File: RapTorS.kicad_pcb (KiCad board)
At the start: 2 copper layers, 45 x 19 mm, 23 parts, among them J1 Molex 48037-2200, J2 TestPoint, J3 TestPoint, J4 TestPoint, J5 TestPoint, J6 TestPoint, U1 PIC16LF1454-I_ML, U2 TLV71333PDBV, U3 E07-M1101S

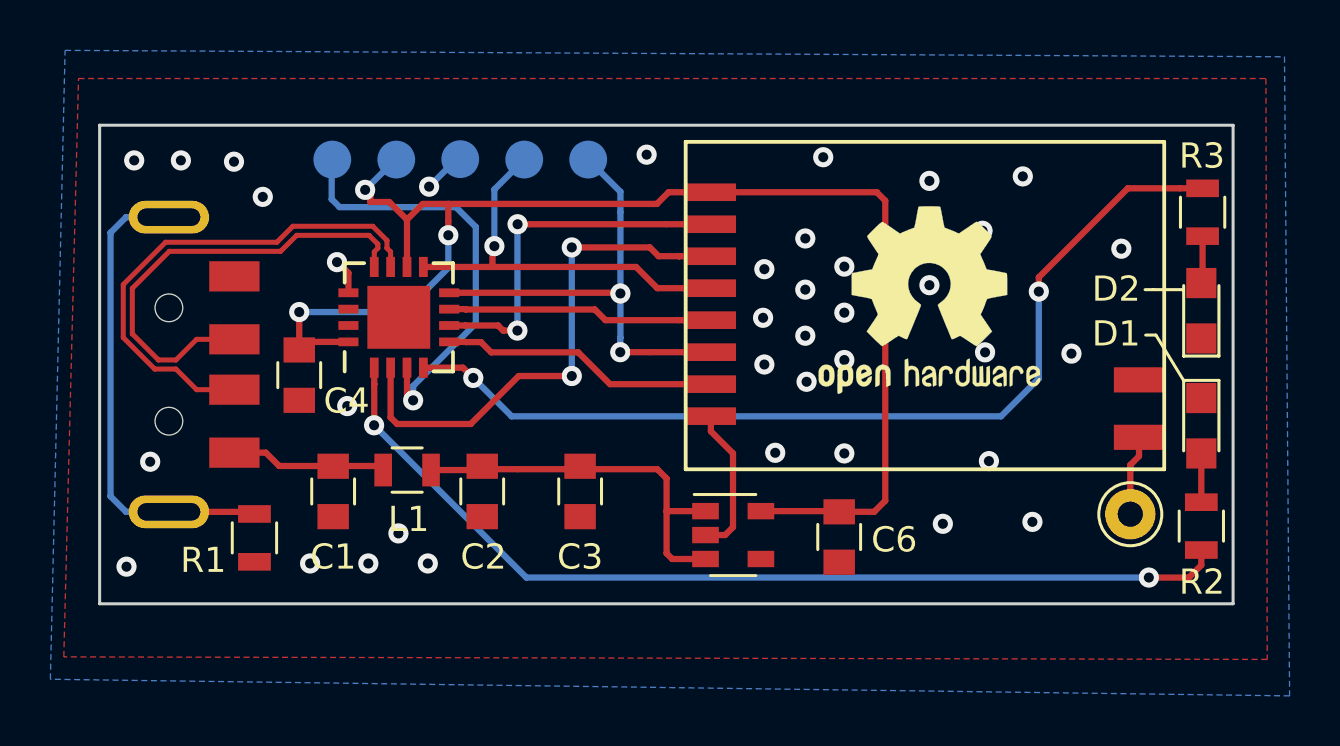
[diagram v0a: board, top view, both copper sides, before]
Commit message: routing completed
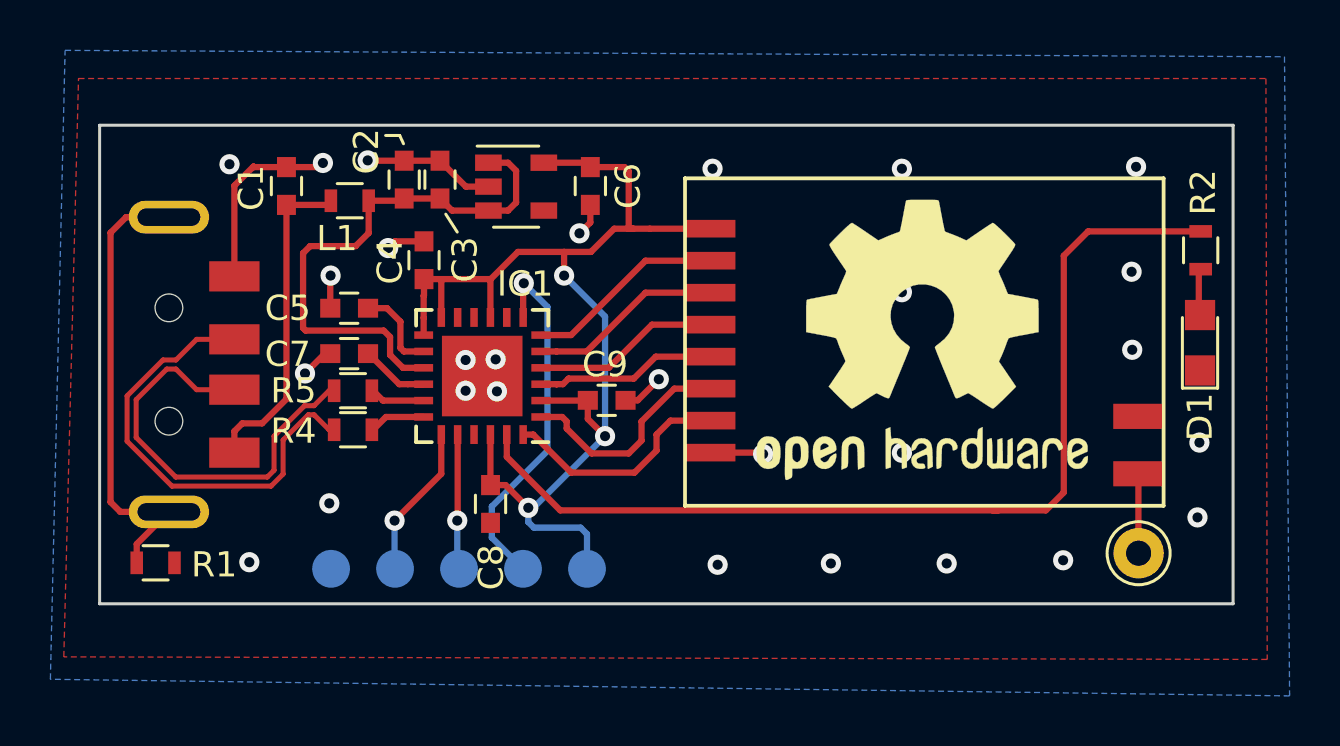
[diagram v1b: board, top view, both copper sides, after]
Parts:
- removed D2: LED_ALT, LEDs:LED_0805
- removed G***: LOGO, Logo:Logo
- removed R3: 50R, Resistors_SMD:R_0805
- removed the REF*** at (171.7, 98.1)
- removed U1: PIC16LF1454-I_ML, Housings_DFN_QFN:QFN-16-1EP_4x4mm_Pitch0.65mm
- added C5: 1uF, Capacitors_SMD:C_0603, F.Cu at (148.7, 98.4)
- added C7: 1uF, Capacitors_SMD:C_0603, F.Cu at (148.7, 100.2)
- added C8: 1uF, Capacitors_SMD:C_0603, F.Cu at (154.3, 106.2)
- added C9: 1uF, Capacitors_SMD:C_0603, F.Cu at (158.9, 102.1)
- added IC1: EFM32HG308F64G-A-QFN24, Housings_DFN_QFN:QFN-24-1EP_5x5mm_Pitch0.65mm, F.Cu at (153.9, 101.1)
- added R4: 15R, Resistors_SMD:R_0603, F.Cu at (148.8, 103.3)
- added R5: 15R, Resistors_SMD:R_0603, F.Cu at (148.8, 101.7)
- added RAPTORS: LOGO, Logo:Logo, B.Cu at (163.1, 100.4)
- added REF***: OSHW-Logo2_14.6x12mm_SilkScreen, Symbols:OSHW-Logo2_14.6x12mm_SilkScreen, F.Cu at (171.4, 99.7)
- C1, C2, C3, C4, C6: footprint Capacitors_SMD:C_0805 -> Capacitors_SMD:C_0603
- L1: footprint Inductors_SMD:L_0805 -> Inductors_SMD:L_0603
- R1, R2: footprint Resistors_SMD:R_0805 -> Resistors_SMD:R_0603
- moved J6 18.0 mm to (150.5, 108.8)
- moved J2 17.9 mm to (155.6, 108.8)
- moved J3 17.9 mm to (158.1, 108.8)
- moved C6 17.1 mm to (158.2, 93.6)
- moved J4 17.1 mm to (147.9, 108.8)
- moved J5 16.5 mm to (153.0, 108.8)
- moved U2 16.3 mm to (155.3, 93.6)
- moved C3 13.6 mm to (152.3, 93.3), turned to 90 degrees
- moved C2 12.8 mm to (150.9, 93.3), turned to 90 degrees
- moved C1 12.3 mm to (146.2, 93.6), turned to 90 degrees
- moved R2 11.0 mm to (182.5, 96.1), turned to 270 degrees
- moved L1 10.9 mm to (148.7, 94.2)
- moved C4 6.73 mm to (151.6, 96.5), turned to 90 degrees
- moved R1 4.05 mm to (141.0, 108.5), turned to 0 degrees
- moved D1 3.29 mm to (182.4, 99.8), turned to 90 degrees
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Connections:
- J2 pad 1: ~MCLR -> ~RESET
- J5 pad 1: ISPDAT -> SWDIO
- J6 pad 1: ISPCLK -> SWCLK
- U2 pad 4: Net-(U2-Pad4) -> (no net)
- U3 pad 4: ISPDAT -> SCK
- U3 pad 6: ISPCLK -> MISO
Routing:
- net LED_DEBUG: track 37.9 -> 0.00 mm, vias 2 -> 0
- net ISPCLK: track 19.2 -> 0.00 mm, vias 2 -> 0
- net ~MCLR: track 16.7 -> 0.00 mm, vias 1 -> 0
- net ISPDAT: track 16.5 -> 0.00 mm, vias 1 -> 0
- net ~RESET: track 0.00 -> 14.5 mm, vias 0 -> 1
- net GND: track 9.10 -> 22.5 mm, vias 37 -> 28
- net CSN: track 20.8 -> 7.69 mm, vias 2 -> 0
- net MISO: track 0.00 -> 9.00 mm
- net +3V3: track 55.3 -> 47.7 mm
- net SCK: track 0.00 -> 7.44 mm
- net Net-(C1-Pad1): track 6.19 -> 13.0 mm
- net GDO0: track 14.7 -> 7.95 mm, vias 2 -> 0
- net +5V: track 15.7 -> 21.9 mm
- net SWCLK: track 0.00 -> 6.11 mm, vias 0 -> 1
- net SWDIO: track 0.00 -> 5.86 mm, vias 0 -> 1
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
